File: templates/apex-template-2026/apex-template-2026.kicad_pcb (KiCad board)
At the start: 2 copper layers, 50 x 50 mm, 0 parts

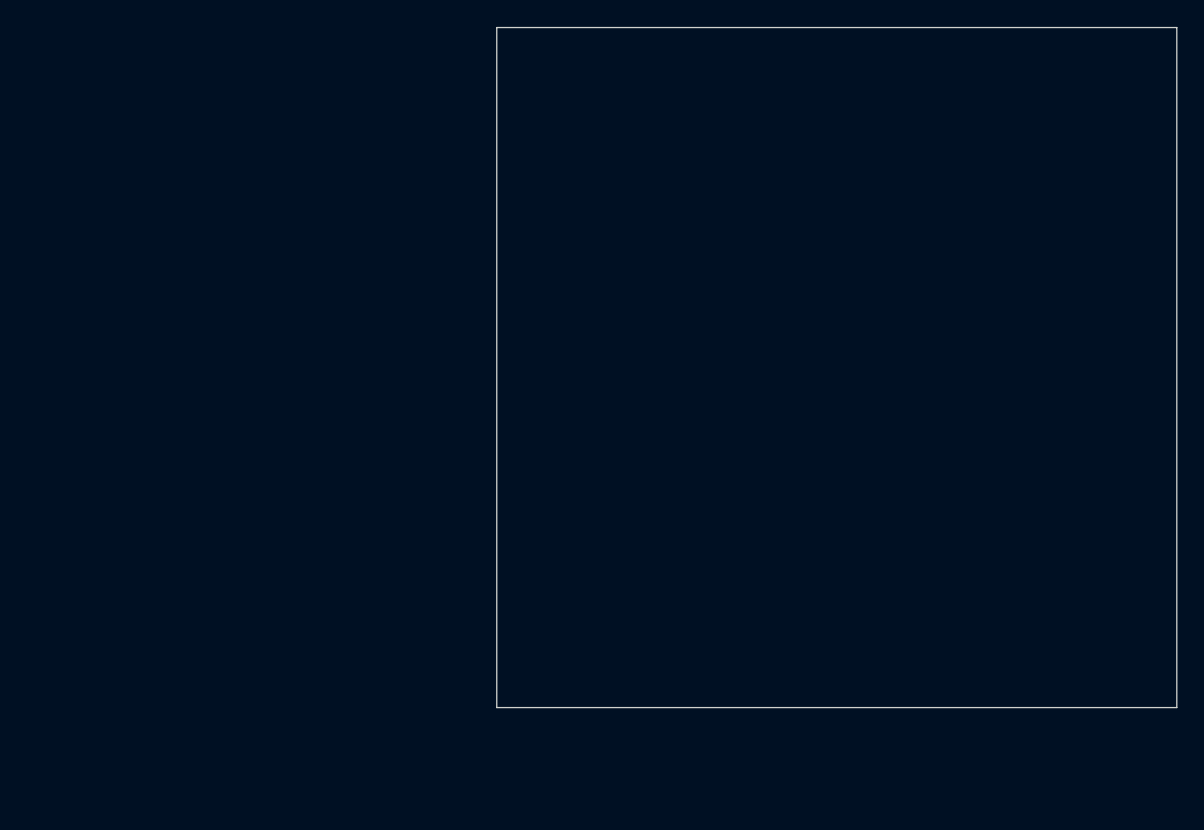
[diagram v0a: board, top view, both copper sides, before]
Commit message: First template version
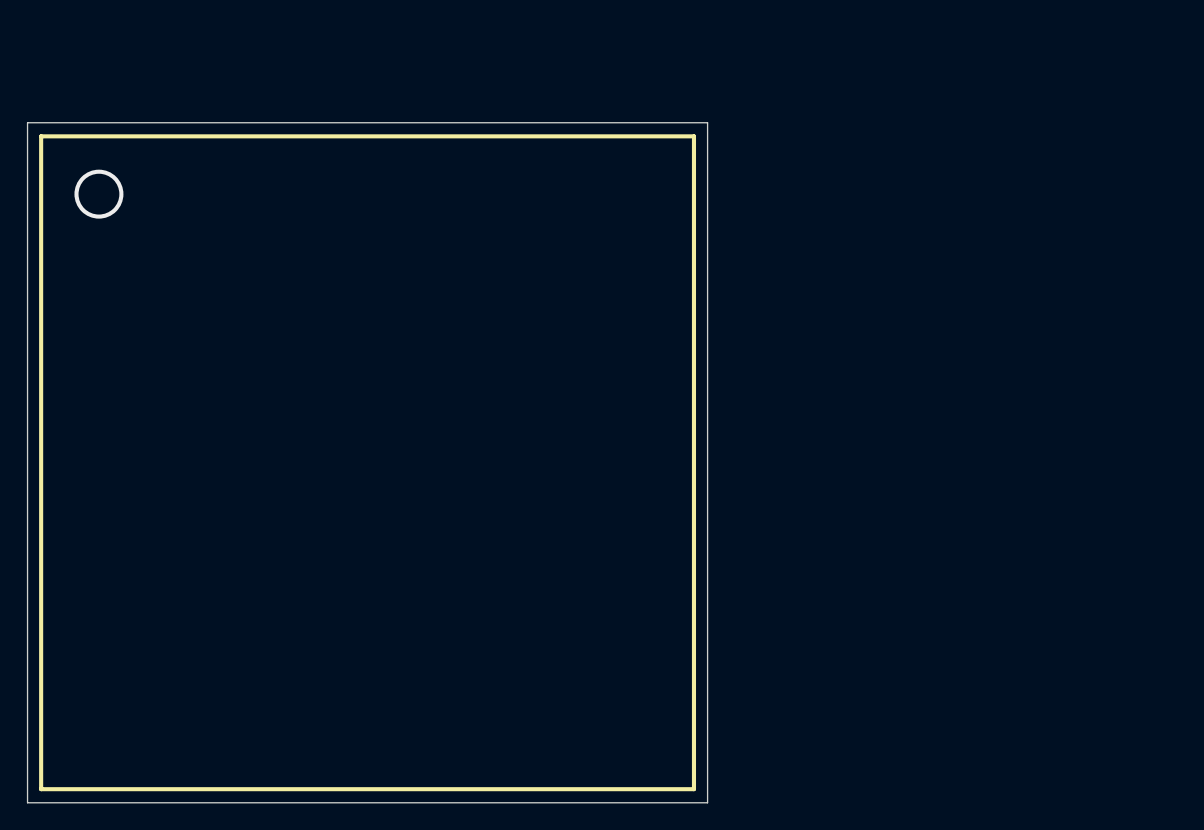
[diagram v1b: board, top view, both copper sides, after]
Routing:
- net (no net): vias 0 -> 1
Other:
- copper layers 2 -> 4
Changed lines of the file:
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@@
 	(generator_version "10.0")
 	(general
-		(thickness 1.6)
+		(thickness 1.6062)
 		(legacy_teardrops no)
 	)
@@
 	(layers
 		(0 "F.Cu" signal)
+		(4 "In1.Cu" power)
+		(6 "In2.Cu" power)
 		(2 "B.Cu" signal)
 		(9 "F.Adhes" user "F.Adhesive")
@@
 	)
 	(setup
+		(stackup
+			(layer "F.SilkS"
+				(type "Top Silk Screen")
+				(color "White")
+			)
+			(layer "F.Paste"
+				(type "Top Solder Paste")
+			)
+			(layer "F.Mask"
+				(type "Top Solder Mask")
+				(color "Green")
+				(thickness 0.01)
+			)
+			(layer "F.Cu"
+				(type "copper")
+				(thickness 0.035)
+			)
+			(layer "dielectric 1"
+				(type "prepreg")
+				(color "FR4 natural")
+				(thickness 0.2104)
+				(material "FR4")
+				(epsilon_r 4.4)
+				(loss_tangent 0.02)
+			)
+			(layer "In1.Cu"
+				(type "copper")
+				(thickness 0.0152)
+			)
+			(layer "dielectric 2"
+				(type "core")
+				(color "FR4 natural")
+				(thickness 1.065)
+				(material "FR4")
+				(epsilon_r 4.6)
+				(loss_tangent 0.02)
+			)
+			(layer "In2.Cu"
+				(type "copper")
+				(thickness 0.0152)
+			)
+			(layer "dielectric 3"
+				(type "prepreg")
+				(color "FR4 natural")
+				(thickness 0.2104)
+				(material "FR4")
+				(epsilon_r 4.4)
+				(loss_tangent 0.02)
+			)
+			(layer "B.Cu"
+				(type "copper")
+				(thickness 0.035)
+			)
+			(layer "B.Mask"
+				(type "Bottom Solder Mask")
+				(color "Green")
+				(thickness 0.01)
+			)
+			(layer "B.Paste"
+				(type "Bottom Solder Paste")
+			)
+			(layer "B.SilkS"
+				(type "Bottom Silk Screen")
+				(color "White")
+			)
+			(copper_finish "HAL SnPb")
+			(dielectric_constraints no)
+		)
 		(pad_to_mask_clearance 0)
 		(allow_soldermask_bridges_in_footprints no)
@@
 		(capping no)
 		(filling no)
+		(zone_defaults)
 		(pcbplotparams
 			(layerselection 0x00000000_00000000_55555555_5755f5ff)
@@
 	)
 	(gr_rect
-		(start 109.5 68)
-		(end 159.5 118)
+		(start 76 76)
+		(end 124 124)
+		(radius 4.5)
+		(stroke
+			(width 0.3)
+			(type solid)
+		)
+		(fill no)
+		(layer "F.SilkS")
+	)
+	(gr_rect
+		(start 75 75)
+		(end 125 125)
 		(radius 5)
 		(stroke
@@
 		(layer "Edge.Cuts")
 	)
+	(via
+		(at 80.25 80.25)
+		(size 3.6)
+		(drill 3)
+		(layers "F.Cu" "B.Cu")
+		(net "")
+	)
 	(embedded_fonts no)
